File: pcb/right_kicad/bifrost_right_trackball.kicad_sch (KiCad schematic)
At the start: 1 part, among them U1 PMW3610

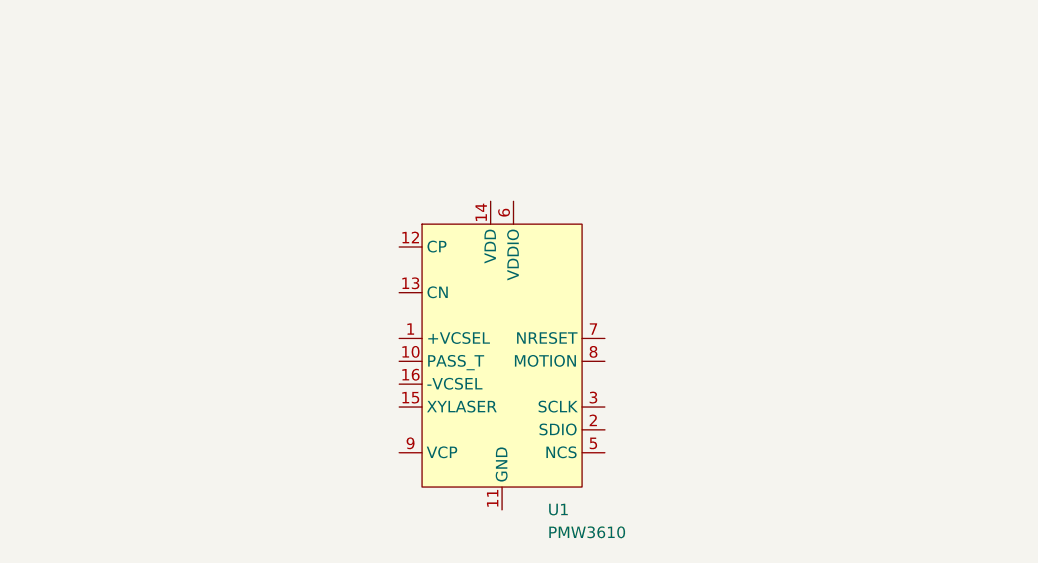
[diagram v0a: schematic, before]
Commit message: Update PCB designs
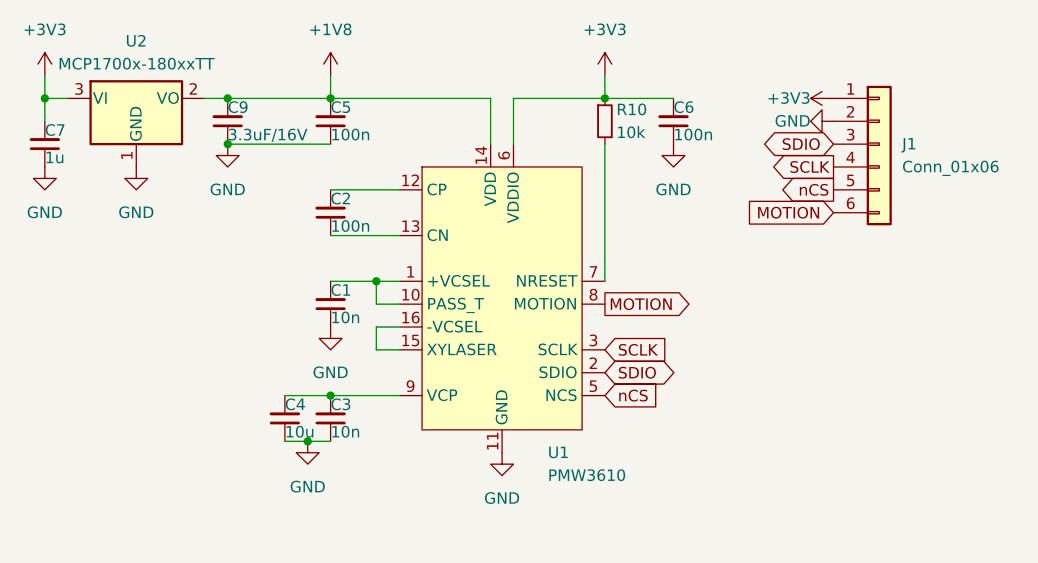
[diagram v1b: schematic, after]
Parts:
- added C1, C3: 10n, Capacitor_SMD:C_0402_1005Metric, symbol Device:C_Small
- added C2, C5, C6: 100n, Capacitor_SMD:C_0402_1005Metric, symbol Device:C_Small
- added C4: 10u, Capacitor_SMD:C_0402_1005Metric, symbol Device:C_Small
- added C7: 1u, Capacitor_SMD:C_0402_1005Metric, symbol Device:C_Small
- added C9: 3.3uF/16V, Capacitor_SMD:C_0603_1608Metric, symbol Device:C_Small
- added J1: Conn_01x06, Connector_PinHeader_1.27mm:PinHeader_1x06_P1.27mm_Vertical, symbol Connector_Generic:Conn_01x06
- added R10: 10k, Resistor_SMD:R_0402_1005Metric, symbol Device:R_Small
- added U2: MCP1700x-180xxTT, Package_TO_SOT_SMD:SOT-23, symbol Regulator_Linear:MCP1700x-180xxTT
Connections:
- net at U1.1 (+VCSEL): now also U1.10 (PASS_T), C1.2
- net GND: now reaches U1.11 (GND)
- net GND: now also C1.1, C3.1, C4.1, C5.1, C6.1, C7.1, C9.1, J1.2 (Pin_2), U2.1 (GND)
- net at U1.12 (CP): now also C2.2
- net at U1.13 (CN): now also C2.1
- net +1V8: now reaches U1.14 (VDD)
- net +1V8: now also C5.2, C9.2, U2.2 (VO)
- net at U1.15 (XYLASER): now also U1.16 (-VCSEL)
- net SDIO: now reaches U1.2 (SDIO)
- net SDIO: now also J1.3 (Pin_3)
- net SCLK: now reaches U1.3 (SCLK)
- net SCLK: now also J1.4 (Pin_4)
- net nCS: now reaches U1.5 (NCS)
- net nCS: now also J1.5 (Pin_5)
- net +3V3: now reaches U1.6 (VDDIO)
- net +3V3: now also C6.2, C7.2, J1.1 (Pin_1), R10.1, U2.3 (VI)
- net at U1.7 (NRESET): now also R10.2
- net MOTION: now reaches U1.8 (MOTION)
- net MOTION: now also J1.6 (Pin_6)
- net at U1.9 (VCP): now also C3.2, C4.2
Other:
- moved on the sheet: U1
